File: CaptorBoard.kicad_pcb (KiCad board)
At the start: 2 copper layers, 65 x 45 mm, 26 parts, among them J1 Conn_01x06, J2 MKDSN 1,5/ 4-5,08, SW1 SKHHLVA010, SW2 SKHHLVA010, U1 WeMos_mini, U2 IRM-02-5, U3 MOC3040X, U4 MOC3040X, U5 DHT22

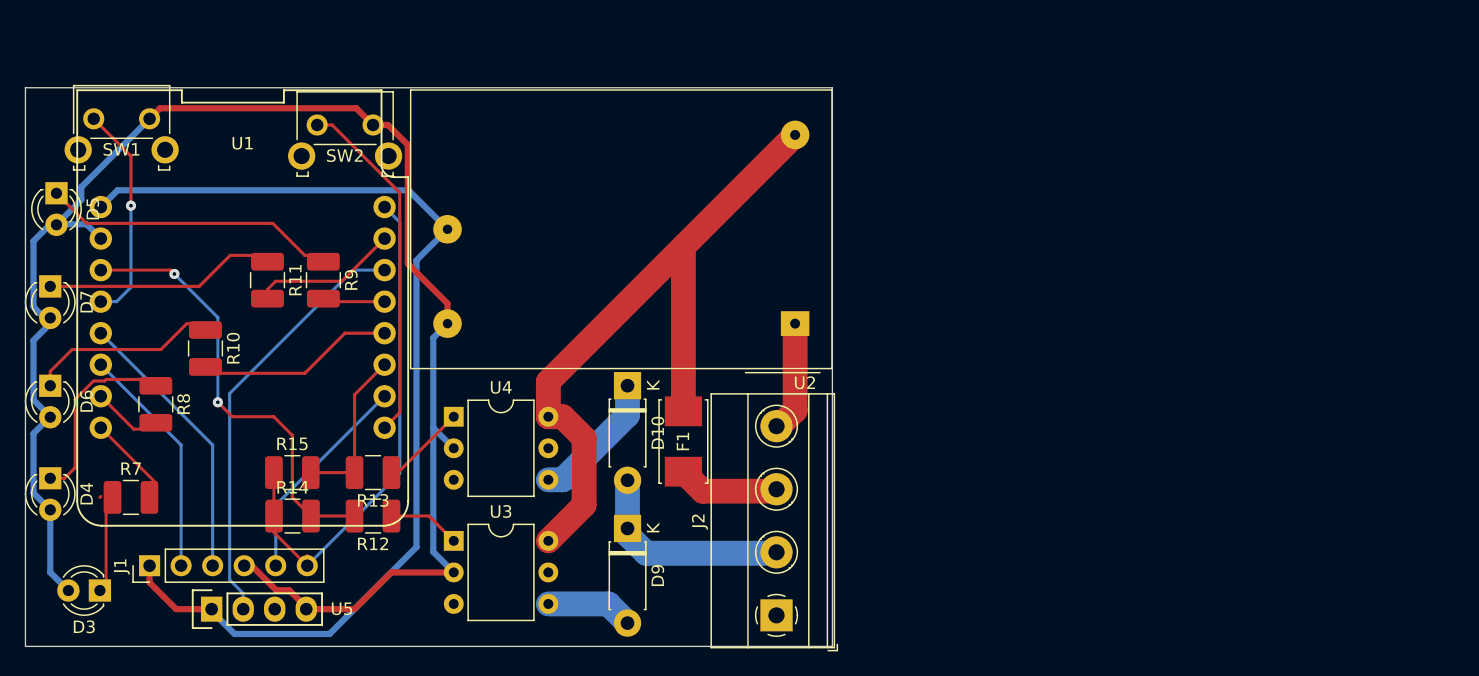
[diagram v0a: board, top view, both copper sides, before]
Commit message: New routing
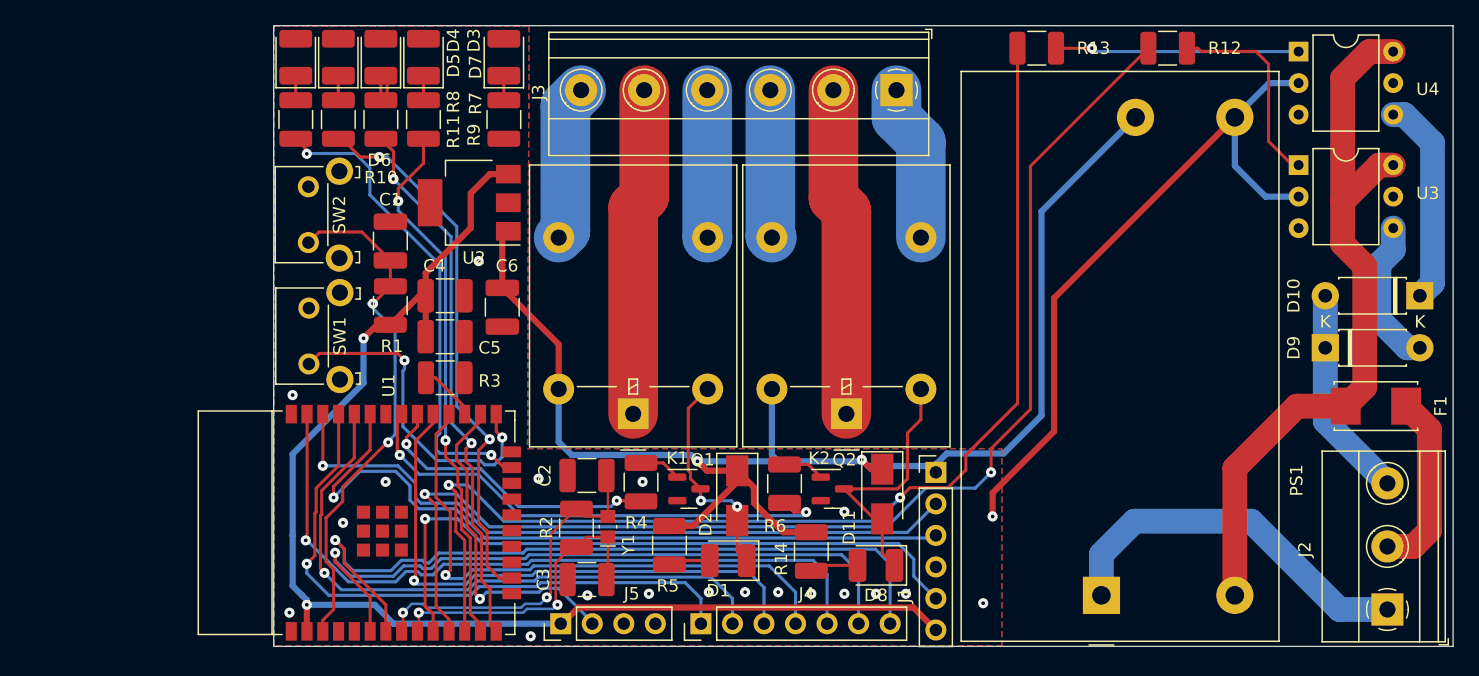
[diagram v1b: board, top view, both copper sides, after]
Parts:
- removed R15: 1k, Resistor_SMD:R_1210_3225Metric_Pad1.42x2.65mm_HandSolder
- removed U5: DHT22, pfo:DHT22_Temperature_Humidity
- added C1: 0.1µ, Capacitor_SMD:C_1210_3225Metric_Pad1.33x2.70mm_HandSolder, F.Cu at (104.4, 67.3)
- added C2: 12p, Capacitor_SMD:C_1210_3225Metric_Pad1.33x2.70mm_HandSolder, F.Cu at (120.2, 86.2)
- added C3: 12p, Capacitor_SMD:C_1210_3225Metric_Pad1.33x2.70mm_HandSolder, F.Cu at (120.2, 94.6)
- added C4: 22µ, Capacitor_SMD:C_1210_3225Metric_Pad1.33x2.70mm_HandSolder, F.Cu at (108.8, 71.8)
- added C5: 0.1µ, Capacitor_SMD:C_1210_3225Metric_Pad1.33x2.70mm_HandSolder, F.Cu at (108.8, 75.1)
- added C6: 1µ, Capacitor_SMD:C_1210_3225Metric_Pad1.33x2.70mm_HandSolder, F.Cu at (113.4, 72.7)
- added D1: REL1, LED_SMD:LED_1210_3225Metric_Pad1.42x2.65mm_HandSolder, F.Cu at (131.6, 93.1)
- added D11: MRA4007T3G, Diode_SMD:D_SMA, F.Cu at (144.0, 87.7)
- added D2: MRA4007T3G, Diode_SMD:D_SMA, F.Cu at (132.3, 87.9)
- added D8: REL2, LED_SMD:LED_1210_3225Metric_Pad1.42x2.65mm_HandSolder, F.Cu at (143.5, 93.5)
- added J3: Screw_Terminal_01x06, TerminalBlock_Phoenix:TerminalBlock_Phoenix_MKDS-1,5-6-5.08_1x06_P5.08mm_Horizontal, F.Cu at (145.2, 55.2)
- added J4: Conn_01x07, Connector_PinHeader_2.54mm:PinHeader_1x07_P2.54mm_Vertical, F.Cu at (129.4, 98.2)
- added J5: Conn_01x04, Connector_PinHeader_2.54mm:PinHeader_1x04_P2.54mm_Vertical, F.Cu at (118.1, 98.2)
- added K1: G5LE-1-DC5, Relay_THT:Relay_SPDT_Omron-G5LE-1, F.Cu at (124.0, 81.3)
- added K2: G5LE-1-DC5, Relay_THT:Relay_SPDT_Omron-G5LE-1, F.Cu at (141.1, 81.3)
- added PS1: IRM-05-5, Converter_ACDC:Converter_ACDC_MeanWell_IRM-05-xx_THT, F.Cu at (161.7, 95.9)
- added Q1: 2N7002E, Package_TO_SOT_SMD:SOT-23, F.Cu at (128.4, 87.3)
- added Q2: 2N7002E, Package_TO_SOT_SMD:SOT-23, F.Cu at (140.0, 87.3)
- added R1: 1k, Resistor_SMD:R_1210_3225Metric_Pad1.30x2.65mm_HandSolder, F.Cu at (104.4, 72.5)
- added R2: 5M, Resistor_SMD:R_1210_3225Metric_Pad1.30x2.65mm_HandSolder, F.Cu at (119.4, 90.5)
- added R3: 10k, Resistor_SMD:R_1210_3225Metric_Pad1.30x2.65mm_HandSolder, F.Cu at (108.8, 78.4)
- added R4: 1k, Resistor_SMD:R_1210_3225Metric_Pad1.30x2.65mm_HandSolder, F.Cu at (124.6, 86.8)
- added R5: 1k, Resistor_SMD:R_1210_3225Metric_Pad1.30x2.65mm_HandSolder, F.Cu at (126.9, 91.8)
- added R6: 1k, Resistor_SMD:R_1210_3225Metric_Pad1.30x2.65mm_HandSolder, F.Cu at (136.1, 86.9)
- added Y1: CM9V-T1A-32.768kHz-7pF-20PPM-TA-QC, Crystal:Crystal_SMD_MicroCrystal_CM9V-T1A-2Pin_1.6x1.0mm_HandSoldering, F.Cu at (121.9, 90.4)
- D3, D4, D5, D6, D7: footprint LED_THT:LED_D3.0mm -> LED_SMD:LED_1210_3225Metric_Pad1.42x2.65mm_HandSolder
- J2: value MKDSN 1,5/ 4-5,08 -> Screw_Terminal_01x03; footprint TerminalBlock_Phoenix:TerminalBlock_Phoenix_MKDS-1,5-4-5.08_1x04_P5.08mm_Horizontal -> TerminalBlock_Phoenix:TerminalBlock_Phoenix_MKDS-1,5-3-5.08_1x03_P5.08mm_Horizontal
- R10, R11, R12, R13, R14, R7, R8, R9: footprint Resistor_SMD:R_1210_3225Metric_Pad1.42x2.65mm_HandSolder -> Resistor_SMD:R_1210_3225Metric_Pad1.30x2.65mm_HandSolder
- U1: value WeMos_mini -> ESP32-WROOM-32E-N4; footprint wemos-d1-mini:wemos-d1-mini-with-pin-header-and-connector -> Espressif:ESP32-WROOM-32E
- U2: value IRM-02-5 -> TC1264-3.3VDBTR; footprint Converter_ACDC:Converter_ACDC_MeanWell_IRM-02-xx_THT -> Package_TO_SOT_SMD:SOT-223-3_TabPin2
- moved U3 74.5 mm to (177.6, 61.2)
- moved R12 74.3 mm to (167.0, 51.8)
- moved U4 74.1 mm to (177.6, 52.1)
- moved D10 64.2 mm to (187.3, 71.8), turned to 180 degrees
- moved J1 63.8 mm to (148.3, 86.0), turned to 0 degrees
- moved R13 63.5 mm to (156.5, 51.8)
- moved D9 58.1 mm to (179.7, 75.9), turned to 0 degrees
- moved F1 55.9 mm to (183.8, 80.6), turned to 0 degrees
- moved D3 53.9 mm to (113.5, 52.5), turned to 90 degrees
- moved J2 49.2 mm to (184.7, 97.0)
- moved D4 45.3 mm to (107.1, 52.5), turned to 90 degrees
- moved R7 42.8 mm to (113.5, 57.6), turned to -90 degrees
- moved R14 41.9 mm to (138.3, 92.4), turned to -90 degrees
- moved D6 37.5 mm to (103.6, 52.5), turned to 90 degrees
- moved R8 31.5 mm to (107.1, 57.6)
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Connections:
- J1 pad 6: +3V3 -> +3.3V
- J2 pad 1: (no net) -> /Neutre
- J2 pad 2: /CMD2 -> /Phase_in
- J2 pad 3: /Phase_in -> /CMD2
- R14 pad 1: +3V3 -> +5V
- R14 pad 2: /PILOT_1 -> Net-(D8-Pad2)
- U1 pad 1: +5V -> GND
- U1 pad 11: /PILOT_2 -> /PILOT_1
- U1 pad 12: /CONF-1°C -> /PILOT_2
- U1 pad 13: /ECO -> /CONF
- U1 pad 14: /CAPTOR -> /CONF-1°C
- U1 pad 15: /CONF-2°C -> GND
- U1 pad 16: +3V3 -> /CONF-2°C
- U1 pad 2: GND -> +3.3V
- U1 pad 3: /PILOT_1 -> /RESET
- U1 pad 4: /SELECT -> unconnected-(U1-Pad4)
- U1 pad 5: /SDA_EXT -> unconnected-(U1-Pad5)
- U1 pad 6: /SCL_EXT -> /GPIO34
- U1 pad 7: /CONF -> /GPIO35
- U1 pad 8: /POWER -> /XP
- U1 pad 9: /RESET -> /XN
- U2 pad 1: /Neutre -> +5V
- U2 pad 2: /Phase -> GND
- U2 pad 3: GND -> +3.3V
- U3 pad 3: (no net) -> unconnected-(U3-Pad3)
- U3 pad 5: (no net) -> unconnected-(U3-Pad5)
- U4 pad 3: (no net) -> unconnected-(U4-Pad3)
- U4 pad 5: (no net) -> unconnected-(U4-Pad5)
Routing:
- net +3.3V: track 0.00 -> 102.2 mm, vias 0 -> 2
- net /PILOT_2: track 13.2 -> 92.6 mm, vias 0 -> 2
- net GND: track 131.1 -> 56.6 mm, vias 0 -> 20
- net /PILOT_1: track 35.6 -> 99.8 mm
- net /GPIO35: track 0.00 -> 61.6 mm, vias 0 -> 1
- net /GPIO23: track 0.00 -> 59.0 mm, vias 0 -> 1
- net /GPIO34: track 0.00 -> 56.5 mm, vias 0 -> 1
- net /RX: track 0.00 -> 50.6 mm, vias 0 -> 1
- net /TX: track 0.00 -> 49.4 mm, vias 0 -> 1
- net /GPIO5: track 0.00 -> 46.2 mm, vias 0 -> 1
- net /GPIO17: track 0.00 -> 46.2 mm, vias 0 -> 1
- net +3V3: track 41.9 -> 0.00 mm
- net /REL2: track 0.00 -> 40.5 mm, vias 0 -> 2
- net /SCL_EXT: track 18.9 -> 57.4 mm, vias 0 -> 1
- net /SDA_EXT: track 22.5 -> 60.4 mm, vias 0 -> 1
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- added copper zone on B.Cu, net GND
- added copper zone on F.Cu, net GND
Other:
- board size 65 x 45 mm -> 95 x 50 mm
- board text added: "1 - 3.3V 2 - Captor 3 - 4 - GND"
- board text added: "1 - 5V 2 - SDC 3 - SDA 4 - GND 5 - Ana 6 - 3.3V"
- board text added: "1 - TX 2 - RX 3 - GPIO5 4 - GPIO17 5 - GPIO23 6 - GPIO34 7 - GPIO35"
- board text added: "CMD"
- board text added: "COM"
- board text added: "Conf -1°C"
- board text added: "Conf -2°C"
- board text added: "Eco"
- board text added: "L"
- board text added: "N"
- board text added: "NC"
- board text added: "NO"
- board text added: "Pwd"
- board text added: "REL 1"
- board text added: "REL 2"
- board text removed: "-1°C"
- board text removed: "-2°C"
- board text removed: "1 - +5V 2 - CAPTEUR 3 - NC 4 - GND"
- board text removed: "1 - +5V 2 - SCL 3 - SDA 4 - GND 5 - ANA 6 - +3.3V"
- board text removed: "1 - Terre 2 - Pilote 3 - Phase 4 - Neutre"
- board text removed: "ECO"
- board text removed: "Reset"
- board text removed: "Select"
- board text removed: "Status"
